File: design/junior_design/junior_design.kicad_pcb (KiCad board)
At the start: 2 copper layers, 28 parts, among them J1 MPLAB SNAP, J2 Screw_Terminal_01x04, J3 Conn_01x05, J4 Conn_01x03, J5 USB_C_Receptacle_USB2.0_16P, U2 INA128, U3 TLV76133DCY, U4 MCP6022

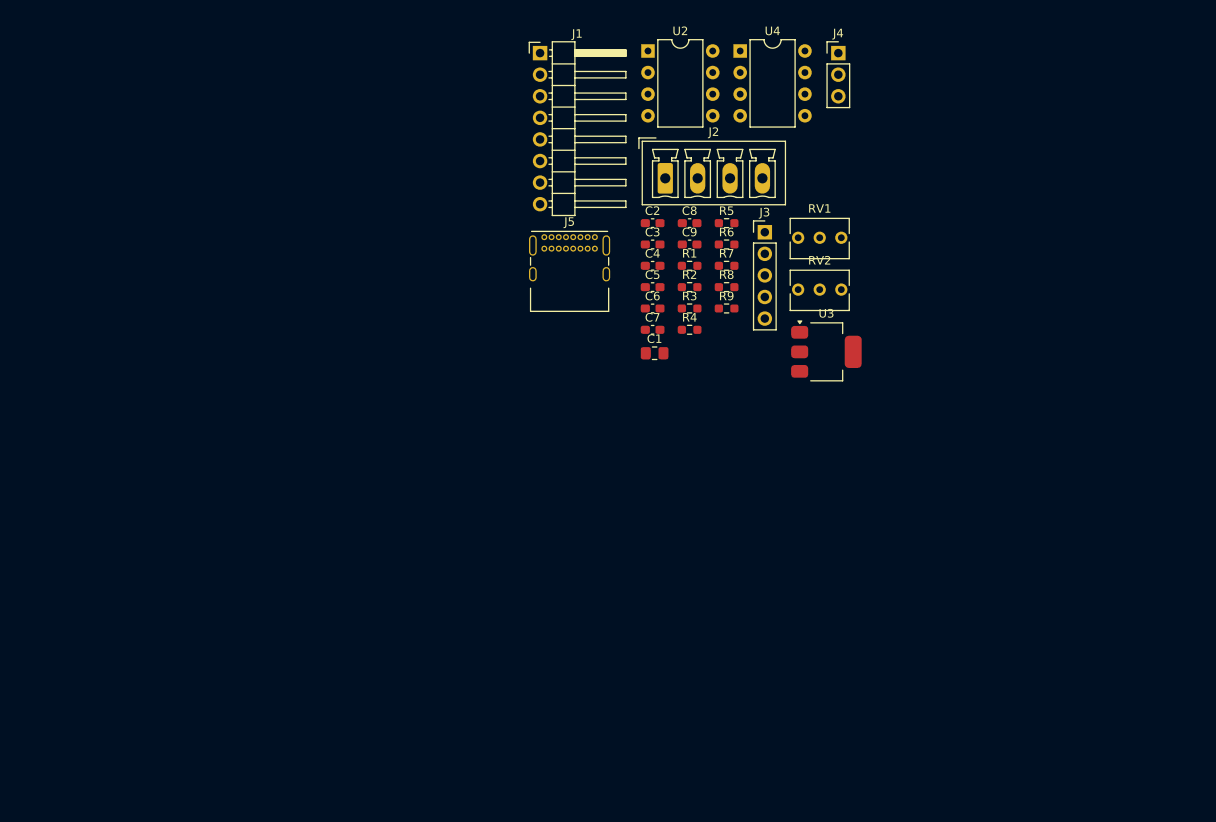
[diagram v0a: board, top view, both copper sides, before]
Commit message: Started PCB layout
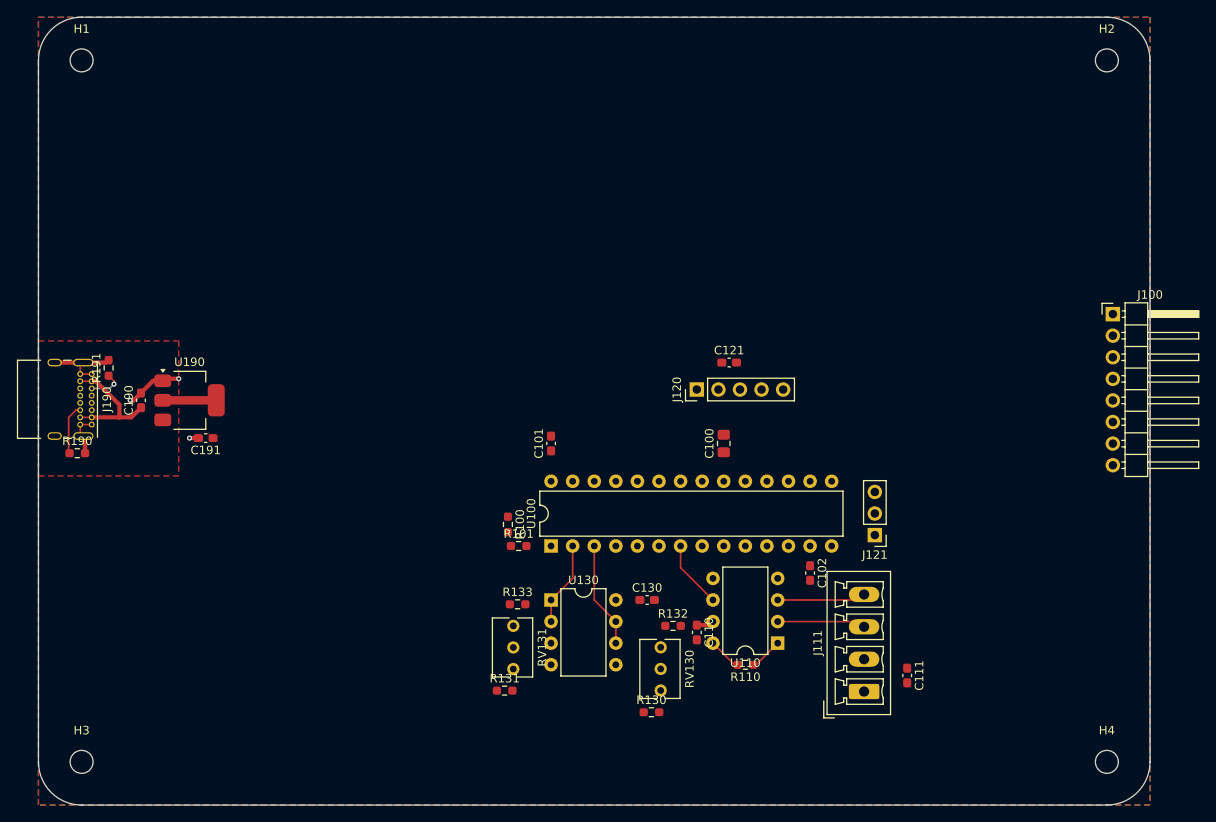
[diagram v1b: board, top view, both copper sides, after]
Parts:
- added H1: MountingHole, MountingHole:MountingHole_2.7mm, F.Cu at (76.2, 76.2)
- added H2: MountingHole, MountingHole:MountingHole_2.7mm, F.Cu at (196.8, 76.2)
- added H3: MountingHole, MountingHole:MountingHole_2.7mm, F.Cu at (76.2, 158.8)
- added H4: MountingHole, MountingHole:MountingHole_2.7mm, F.Cu at (196.8, 158.8)
- added U100: PIC24FJ64GA002-I_SP, Package_DIP:DIP-28_W7.62mm, F.Cu at (131.4, 133.3)
- moved R190 78.9 mm to (75.7, 122.4)
- moved U190 75.2 mm to (88.9, 116.2)
- moved J100 74.1 mm to (197.6, 106.1)
- moved R191 73.1 mm to (79.4, 112.4), turned to 90 degrees
- moved U110 71.3 mm to (158.1, 144.8), turned to 180 degrees
- moved U130 68.3 mm to (131.4, 139.7)
- moved J111 64.8 mm to (168.3, 150.5), turned to 90 degrees
- moved RV131 63.8 mm to (127.0, 147.8), turned to -90 degrees
- moved C190 62.3 mm to (83.2, 116.2), turned to 90 degrees
- moved J121 56.9 mm to (169.5, 132.1), turned to 180 degrees
- moved J190 55.6 mm to (77.4, 113.1), turned to -90 degrees
- moved C191 55.5 mm to (90.8, 120.7), turned to 180 degrees
- moved C111 52.6 mm to (173.4, 148.6), turned to -90 degrees
- moved RV130 51.7 mm to (144.3, 150.4), turned to -90 degrees
- moved R133 51.2 mm to (127.5, 140.2)
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- renumbered C1 to C100, C2 to C101, C3 to C102, C7 to C110, C6 to C111, C9 to C121, C8 to C130, C4 to C190, C5 to C191, J1 to J100, J2 to J111, J3 to J120, J4 to J121, J5 to J190, R7 to R100, R6 to R101, R1 to R110, R2 to R130, R4 to R131, R3 to R132, R5 to R133, R8 to R190, R9 to R191, RV2 to RV130, RV1 to RV131, U2 to U110, U4 to U130, U3 to U190
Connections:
- J190 pad S1: unconnected-(J5-SHIELD-PadS1) -> GND
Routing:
- net GND: track 0.00 -> 22.1 mm, vias 0 -> 3
- net +5V: track 0.00 -> 14.9 mm
- net Net-(U100-AN1/VREF-/CN3/RA1): track 0.00 -> 12.5 mm
- net /LDCELL+: track 0.00 -> 10.4 mm
- net /LDCELL-: track 0.00 -> 10.4 mm
- net Net-(U100-AN0/VREF+/CN2/RA0): track 0.00 -> 9.94 mm
- net +3.3V: track 0.00 -> 8.37 mm
- net Net-(U100-AN5/C1IN+/RP3/SCL2/CN7/RB3): track 0.00 -> 7.93 mm
- net Net-(J190-CC2): track 0.00 -> 5.96 mm
- net Net-(J190-CC1): track 0.00 -> 4.09 mm, vias 0 -> 1
- net Net-(R110-Pad2): track 0.00 -> 3.96 mm
- net Net-(R110-Pad1): track 0.00 -> 3.94 mm
- added copper zone on F.Cu, net +3.3V
- added copper zone on F.Cu, net +5V
- added copper zone on B.Cu, net GND
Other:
- board outline added: 130.8 x 92.7 mm
